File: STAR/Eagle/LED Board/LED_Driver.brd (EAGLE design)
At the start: 20.3 x 10.4 mm, 9 parts

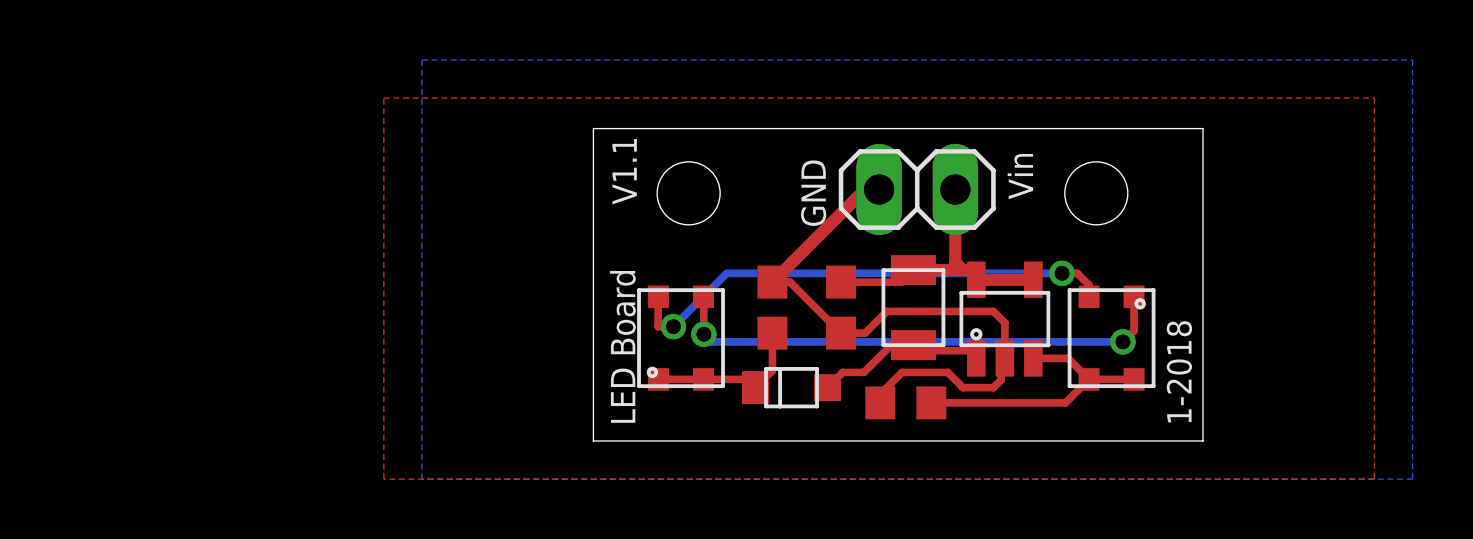
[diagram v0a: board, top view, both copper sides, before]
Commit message: CAD for STARduino, datalogger
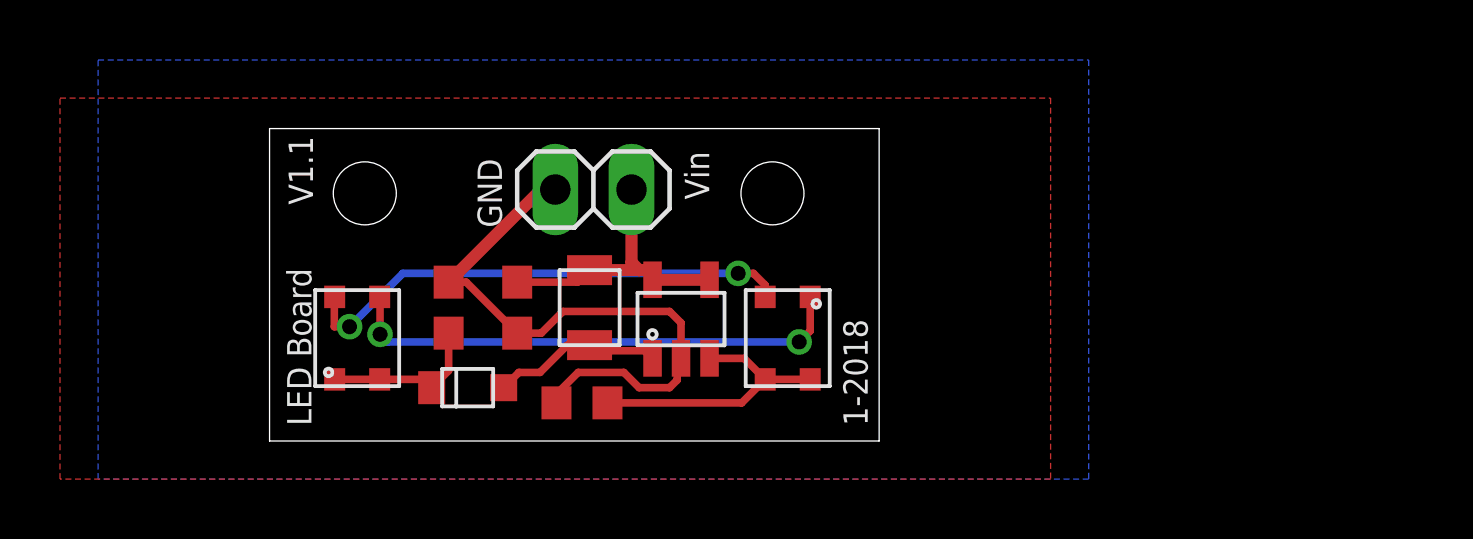
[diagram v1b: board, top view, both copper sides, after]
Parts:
- moved U$2 10.8 mm to (10.7, 4.45)
- moved U$3 10.8 mm to (6.60, 1.78)
- moved U$5 10.8 mm to (17.3, 3.43)
- moved C2 10.8 mm to (8.26, 4.45)
- moved JP1 10.8 mm to (10.8, 8.38)
- moved R1 10.8 mm to (10.4, 1.27)
- moved U$1 10.8 mm to (13.7, 4.06)
- moved U$4 10.8 mm to (2.92, 3.43)
- moved C1 10.8 mm to (5.97, 4.45)
